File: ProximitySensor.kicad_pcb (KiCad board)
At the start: 2 copper layers, 45 x 17 mm, 17 parts, among them Q1 Q_PMOS_GSD, Q2 Q_NMOS_GSD, U1 L78L05_SOT89, U2 LM393, X1 CONN_3

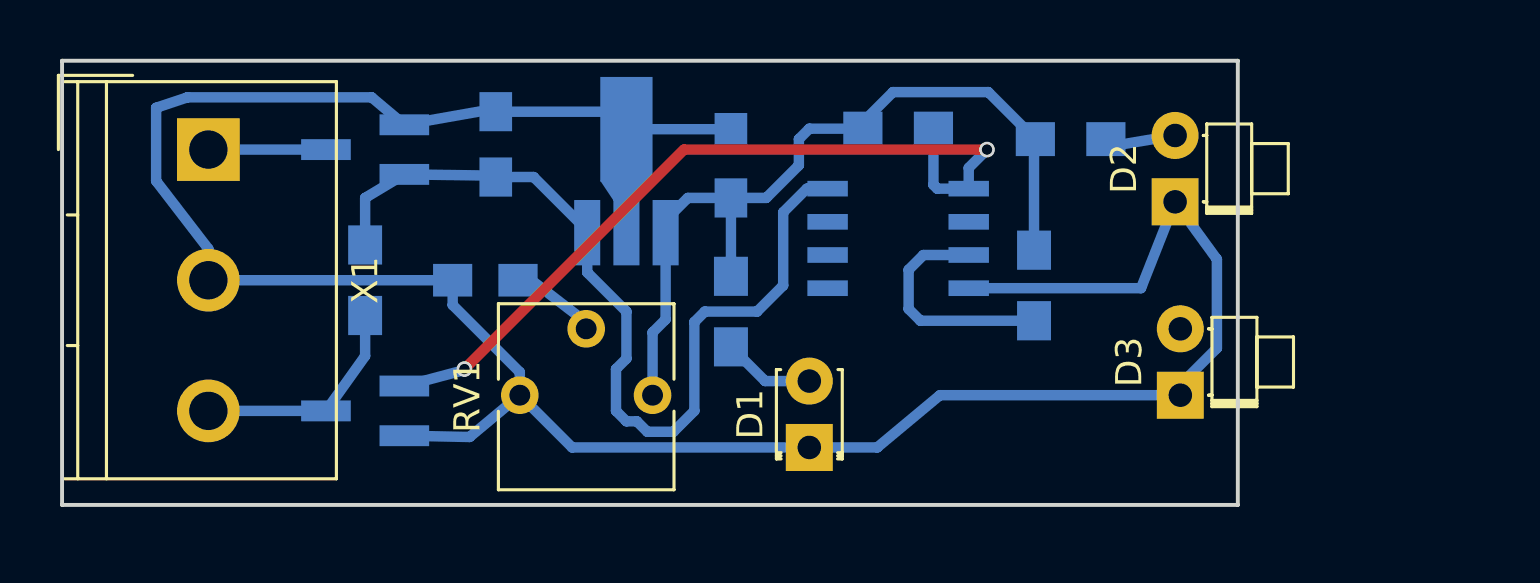
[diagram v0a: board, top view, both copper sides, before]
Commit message: New topology
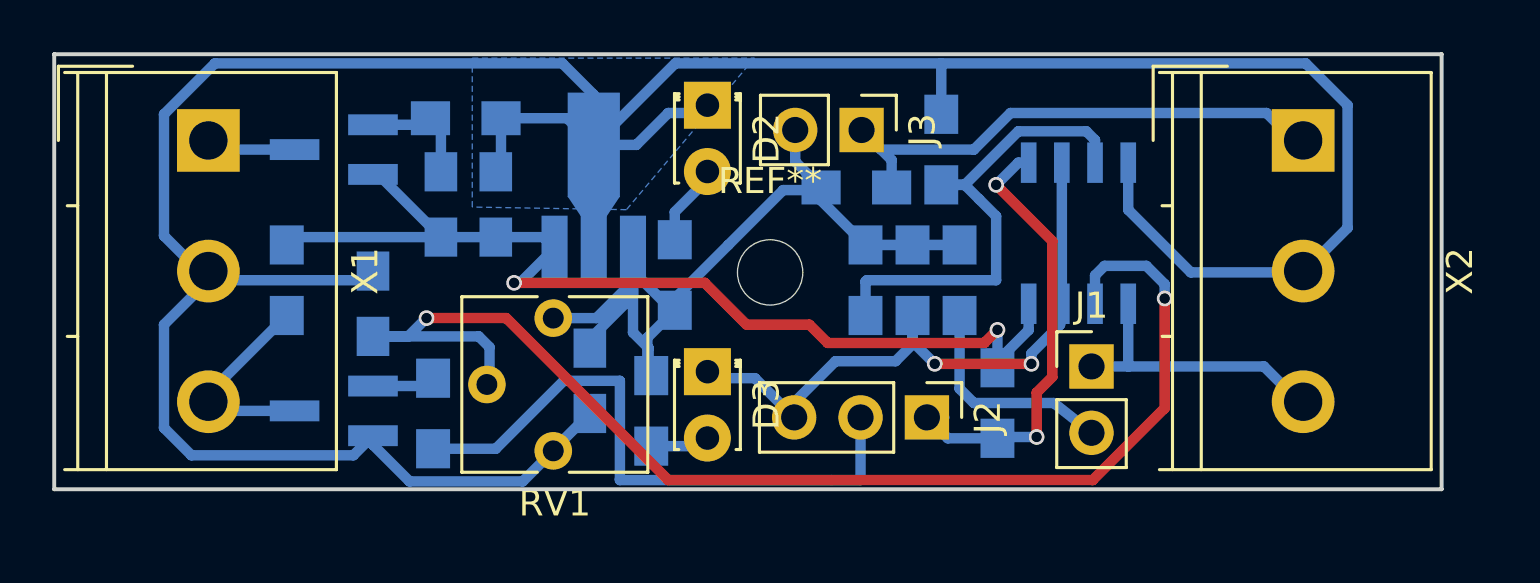
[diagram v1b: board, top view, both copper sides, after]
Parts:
- added J1: Conn_01x02_Male, Pin_Headers:Pin_Header_Straight_1x02_Pitch2.54mm, F.Cu at (157.2, 111.7)
- added J2: Conn_01x03_Male, Pin_Headers:Pin_Header_Straight_1x03_Pitch2.54mm, F.Cu at (150.9, 113.7)
- added J3: Conn_01x02_Male, Pin_Headers:Pin_Header_Straight_1x02_Pitch2.54mm, F.Cu at (148.4, 102.7)
- added R10: 5k, Resistors_SMD:R_0805_HandSoldering, B.Cu at (126.4, 108.4)
- added R11: 470R, Resistors_SMD:R_0805_HandSoldering, B.Cu at (148.2, 104.8)
- added R6: 5k, Resistors_SMD:R_0805_HandSoldering, B.Cu at (148.6, 108.4)
- added R7: 5k, Resistors_SMD:R_0805_HandSoldering, B.Cu at (151.4, 103.4)
- added R8: 5k, Resistors_SMD:R_0805_HandSoldering, B.Cu at (153.6, 113.1)
- added R9: 100R, Resistors_SMD:R_0805_HandSoldering, B.Cu at (132.0, 113.5)
- added REF**: MountingHole_2.5mm, Mounting_Holes:MountingHole_2.5mm, F.Cu at (144.9, 108.1)
- added X2: CONN_3, Connectors_Terminal_Blocks:TerminalBlock_Philmore_TB133_03x5mm_Straight, F.Cu at (165.3, 103.0)
- C3: value C -> 100nF
- D1: value LED_ALT -> D_Zener; footprint LEDs:LED_D1.8mm_W3.3mm_H2.4mm -> Capacitors_SMD:C_0805_HandSoldering; moved to B.Cu
- D2: value LED_ALT -> LED_POWER; footprint LEDs:LED_D1.8mm_W1.8mm_H2.4mm_Horizontal_O1.27mm_Z8.2mm -> LEDs:LED_D1.8mm_W3.3mm_H2.4mm
- D3: value BP104 -> LED_SIGNAL; footprint LEDs:LED_D1.8mm_W1.8mm_H2.4mm_Horizontal_O1.27mm_Z8.2mm -> LEDs:LED_D1.8mm_W3.3mm_H2.4mm
- R1: value 470R -> 100k
- R4: value R -> 5k
- R5: value R -> 470R
- moved D2 18.3 mm to (142.5, 101.7), turned to 270 degrees
- moved D3 18.1 mm to (142.5, 111.9), turned to 270 degrees
- moved D1 16.9 mm to (132.3, 105.5)
- moved R2 16.0 mm to (141.2, 108.2), turned to 90 degrees
- moved R1 12.6 mm to (133.2, 102.2), turned to 0 degrees
- moved R5 12.0 mm to (140.3, 113.4)
- moved C2 9.86 mm to (138.0, 112.2), turned to 270 degrees
- moved U2 6.90 mm to (156.7, 106.6), turned to 270 degrees
- moved R4 5.83 mm to (150.3, 108.4), turned to 270 degrees
- moved RV1 4.81 mm to (136.6, 109.8), turned to 180 degrees
- moved C3 4.39 mm to (129.7, 109.3), turned to 90 degrees
- moved R3 2.86 mm to (152.2, 108.4)
- moved C1 2.30 mm to (134.4, 105.5)
- moved U1 1.39 mm to (138.2, 105.2)
- moved Q1 1.20 mm to (128.2, 103.4)
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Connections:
- C1 pad 1: Net-(C1-Pad1) -> /Vcc
- D1 pad 1: /Gnd -> /Vcc
- D3 pad 1: /Gnd -> Net-(D3-Pad1)
- Q1 pad 1: /Gnd -> Net-(D1-Pad2)
- Q1 pad 2: Net-(C1-Pad1) -> /Vcc
- R1 pad 1: /5v -> Net-(D1-Pad2)
- R1 pad 2: Net-(D1-Pad2) -> /Gnd
- R3 pad 2: Net-(D3-Pad2) -> Net-(J1-Pad2)
- R4 pad 1: Net-(Q2-Pad1) -> /5v
- R4 pad 2: /5v -> Net-(D3-Pad1)
- R5 pad 1: Net-(C1-Pad1) -> /5v
- R5 pad 2: Net-(Q2-Pad3) -> Net-(D3-Pad2)
- U1 pad 3: Net-(C1-Pad1) -> /Vcc
- U2 pad 1: Net-(Q2-Pad1) -> Net-(J2-Pad1)
- U2 pad 2: Net-(U2-Pad2) -> Net-(D3-Pad1)
- U2 pad 3: Net-(D3-Pad2) -> Net-(R6-Pad2)
- U2 pad 5: (no net) -> /sign
- U2 pad 6: (no net) -> Net-(C3-Pad1)
- U2 pad 7: (no net) -> Net-(D3-Pad1)
- U2 pad 8: Net-(C1-Pad1) -> /Vcc
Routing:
- net Net-(C3-Pad1): track 3.54 -> 49.4 mm, vias 0 -> 2
- net /Vcc: track 0.00 -> 40.4 mm, vias 0 -> 2
- net Net-(C1-Pad1): track 35.2 -> 0.00 mm
- net Net-(Q2-Pad1): track 31.2 -> 2.42 mm, vias 2 -> 0
- net Net-(D3-Pad1): track 0.00 -> 25.1 mm, vias 0 -> 2
- net Net-(J2-Pad2): track 0.00 -> 23.6 mm
- net Net-(J3-Pad1): track 0.00 -> 21.0 mm
- net Net-(R6-Pad2): track 0.00 -> 19.1 mm
- net Net-(J2-Pad1): track 0.00 -> 17.7 mm, vias 0 -> 2
- net /Gnd: track 101.6 -> 118.8 mm
- net /sign: track 0.00 -> 11.3 mm
- net Net-(J1-Pad2): track 0.00 -> 8.47 mm
- net Net-(D3-Pad2): track 9.02 -> 2.47 mm
- net /5v: track 31.8 -> 38.3 mm
- net Net-(D1-Pad2): track 3.54 -> 5.23 mm
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- added copper zone on B.Cu, net /Gnd
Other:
- board size 45 x 17 mm -> 53.1 x 16.7 mm
- net class small added: clearance 0.25, trace_width 0.3, via_dia 0.6, via_drill 0.4
